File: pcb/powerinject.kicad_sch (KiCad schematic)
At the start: 3 parts, among them J1 PC_Usb, J2 Charger_USB, J3 Phone_USB

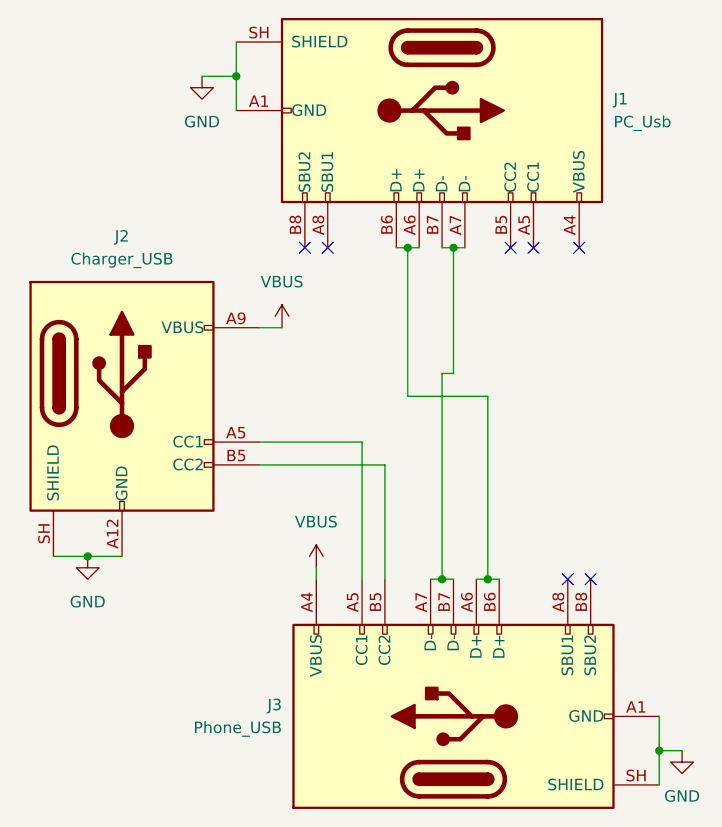
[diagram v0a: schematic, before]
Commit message: make pcb
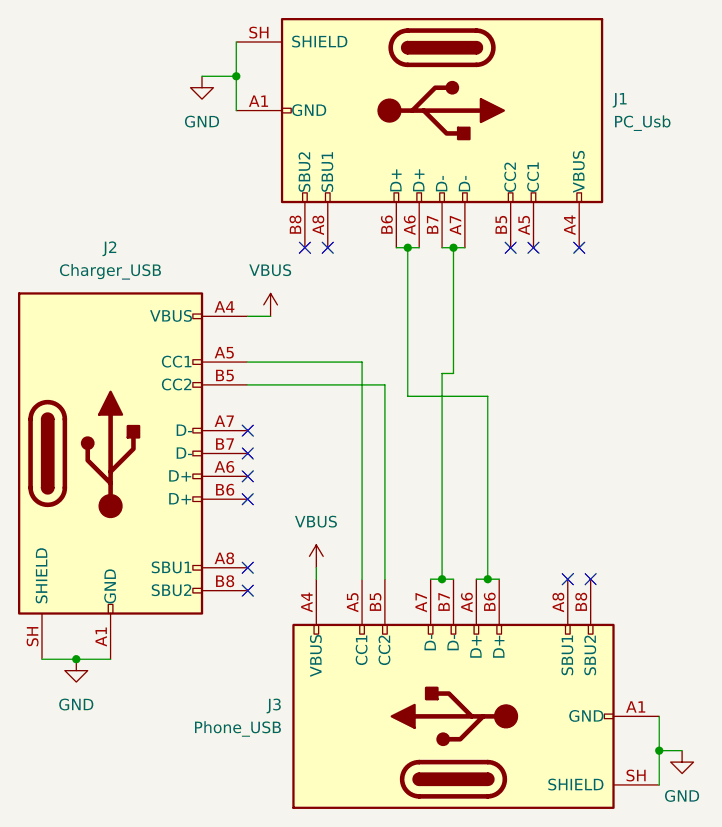
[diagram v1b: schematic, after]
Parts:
- J2: symbol Connector:USB_C_Receptacle_PowerOnly_6P -> Connector:USB_C_Receptacle_USB2.0_16P
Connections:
- net GND: now also J2.A1 (GND), J2.B1 (GND)
- net VBUS: now also J2.A4 (VBUS), J2.B4 (VBUS)
- no-connect marks 7 -> 13
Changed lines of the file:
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@@
+	)
+	(junction
+		(at 55.88 85.09)
+		(diameter 0)
+		(color 0 0 0 0)
 	)
 	(junction
@@
 		(color 0 0 0 0)
 	)
-	(junction
-		(at 57.15 73.66)
-		(diameter 0)
-		(color 0 0 0 0)
+	(no_connect
+		(at 74.93 62.23)
+	)
+	(no_connect
+		(at 74.93 64.77)
+	)
+	(no_connect
+		(at 74.93 77.47)
 	)
 	(no_connect
@@
 	)
 	(no_connect
+		(at 74.93 67.31)
+	)
+	(no_connect
 		(at 110.49 76.2)
 	)
@@
 	)
 	(no_connect
+		(at 74.93 59.69)
+	)
+	(no_connect
 		(at 104.14 39.37)
 	)
 	(no_connect
+		(at 74.93 74.93)
+	)
+	(no_connect
 		(at 106.68 39.37)
 	)
@@
 	(wire
 		(pts
-			(xy 53.34 73.66) (xy 57.15 73.66)
-		)
-		(stroke
-			(width 0)
-			(type default)
-		)
-	)
-	(wire
-		(pts
 			(xy 120.65 95.25) (xy 120.65 99.06)
 		)
@@
 	(wire
 		(pts
-			(xy 87.63 60.96) (xy 76.2 60.96)
-		)
-		(stroke
-			(width 0)
-			(type default)
-		)
-	)
-	(wire
-		(pts
-			(xy 90.17 63.5) (xy 76.2 63.5)
-		)
-		(stroke
-			(width 0)
-			(type default)
-		)
-	)
-	(wire
-		(pts
 			(xy 95.25 76.2) (xy 96.52 76.2)
 		)
@@
 	(wire
 		(pts
+			(xy 55.88 85.09) (xy 59.69 85.09)
+		)
+		(stroke
+			(width 0)
+			(type default)
+		)
+	)
+	(wire
+		(pts
 			(xy 101.6 55.88) (xy 101.6 76.2)
 		)
@@
 	(wire
 		(pts
+			(xy 74.93 46.99) (xy 77.47 46.99)
+		)
+		(stroke
+			(width 0)
+			(type default)
+		)
+	)
+	(wire
+		(pts
 			(xy 97.79 39.37) (xy 99.06 39.37)
 		)
@@
 	(wire
 		(pts
+			(xy 74.93 54.61) (xy 90.17 54.61)
+		)
+		(stroke
+			(width 0)
+			(type default)
+		)
+	)
+	(wire
+		(pts
 			(xy 73.66 16.51) (xy 73.66 20.32)
 		)
@@
 	(wire
 		(pts
-			(xy 76.2 48.26) (xy 78.74 48.26)
-		)
-		(stroke
-			(width 0)
-			(type default)
-		)
-	)
-	(wire
-		(pts
 			(xy 96.52 53.34) (xy 96.52 76.2)
 		)
@@
 	(wire
 		(pts
-			(xy 90.17 76.2) (xy 90.17 63.5)
+			(xy 90.17 54.61) (xy 90.17 76.2)
 		)
 		(stroke
@@
 	(wire
 		(pts
-			(xy 87.63 76.2) (xy 87.63 60.96)
-		)
-		(stroke
-			(width 0)
-			(type default)
-		)
-	)
-	(wire
-		(pts
-			(xy 57.15 73.66) (xy 60.96 73.66)
+			(xy 87.63 52.07) (xy 74.93 52.07)
+		)
+		(stroke
+			(width 0)
+			(type default)
+		)
+	)
+	(wire
+		(pts
+			(xy 87.63 52.07) (xy 87.63 76.2)
 		)
 		(stroke
@@
 		)
 	)
+	(wire
+		(pts
+			(xy 52.07 85.09) (xy 55.88 85.09)
+		)
+		(stroke
+			(width 0)
+			(type default)
+		)
+	)
 	(symbol
-		(lib_id "Connector:USB_C_Receptacle_PowerOnly_6P")
-		(at 60.96 55.88 0)
+		(lib_id "Connector:USB_C_Receptacle_USB2.0_16P")
+		(at 59.69 62.23 0)
 		(unit 1)
 		(body_style 1)
@@
 		(fields_autoplaced yes)
 		(property "Reference" "J2"
-			(at 60.96 38.1 0)
+			(at 59.69 39.37 0)
 			(show_name no)
 			(do_not_autoplace no)
@@
 		)
 		(property "Value" "Charger_USB"
-			(at 60.96 40.64 0)
+			(at 59.69 41.91 0)
 			(show_name no)
 			(do_not_autoplace no)
@@
 		)
 		(property "Footprint" "Connector_USB:USB_C_Receptacle_HRO_TYPE-C-31-M-12"
-			(at 64.77 53.34 0)
+			(at 63.5 62.23 0)
 			(hide yes)
 			(show_name no)
@@
 		)
 		(property "Datasheet" "https://www.usb.org/sites/default/files/documents/usb_type-c.zip"
-			(at 60.96 55.88 0)
-			(hide yes)
-			(show_name no)
-			(do_not_autoplace no)
-			(effects
-				(font
-					(size 1.27 1.27)
-				)
-			)
-		)
-		(property "Description" "USB Power-Only 6P Type-C Receptacle connector"
-			(at 60.96 55.88 0)
+			(at 63.5 62.23 0)
+			(hide yes)
+			(show_name no)
+			(do_not_autoplace no)
+			(effects
+				(font
+					(size 1.27 1.27)
+				)
+			)
+		)
+		(property "Description" "USB 2.0-only 16P Type-C Receptacle connector"
+			(at 59.69 62.23 0)
 			(hide yes)
 			(show_name no)
@@
 		)
 		(property "AliExpress Link" "https://pt.aliexpress.com/item/1005007419369264.html"
-			(at 60.96 55.88 0)
+			(at 59.69 62.23 0)
 			(hide yes)
 			(show_name no)
@@
 		)
 		(property "Price" "US $1.24"
-			(at 60.96 55.88 0)
+			(at 59.69 62.23 0)
 			(hide yes)
 			(show_name no)
@@
 		)
 		(pin "B12"
+		)
+		(pin "B6"
+		)
+		(pin "B8"
+		)
+		(pin "A6"
+		)
+		(pin "B1"
+		)
+		(pin "A1"
+		)
+		(pin "A4"
+		)
+		(pin "A7"
+		)
+		(pin "B7"
+		)
+		(pin "A8"
+		)
+		(pin "B4"
 		)
 		(instances
@@
 	(symbol
 		(lib_id "power:VBUS")
-		(at 78.74 48.26 0)
+		(at 77.47 46.99 0)
 		(unit 1)
 		(body_style 1)
@@
 		(fields_autoplaced yes)
 		(property "Reference" "#PWR02"
-			(at 78.74 52.07 0)
+			(at 77.47 50.8 0)
 			(hide yes)
 			(show_name no)
@@
 		)
 		(property "Value" "VBUS"
-			(at 78.74 43.18 0)
+			(at 77.47 41.91 0)
 			(show_name no)
 			(do_not_autoplace no)
@@
 		)
 		(property "Footprint" ""
-			(at 78.74 48.26 0)
+			(at 77.47 46.99 0)
 			(hide yes)
 			(show_name no)
@@
 		)
 		(property "Datasheet" ""
-			(at 78.74 48.26 0)
+			(at 77.47 46.99 0)
 			(hide yes)
 			(show_name no)
@@
 		)
 		(property "Description" "Power symbol creates a global label with name \"VBUS\""
-			(at 78.74 48.26 0)
+			(at 77.47 46.99 0)
 			(hide yes)
 			(show_name no)
@@
 	(symbol
 		(lib_id "power:GND")
-		(at 57.15 73.66 0)
+		(at 55.88 85.09 0)
 		(unit 1)
 		(body_style 1)
@@
 		(fields_autoplaced yes)
 		(property "Reference" "#PWR03"
-			(at 57.15 80.01 0)
+			(at 55.88 91.44 0)
 			(hide yes)
 			(show_name no)
@@
 		)
 		(property "Value" "GND"
-			(at 57.15 78.74 0)
+			(at 55.88 90.17 0)
 			(show_name no)
 			(do_not_autoplace no)
@@
 		)
 		(property "Footprint" ""
-			(at 57.15 73.66 0)
+			(at 55.88 85.09 0)
 			(hide yes)
 			(show_name no)
@@
 		)
 		(property "Datasheet" ""
-			(at 57.15 73.66 0)
+			(at 55.88 85.09 0)
 			(hide yes)
 			(show_name no)
@@
 		)
 		(property "Description" "Power symbol creates a global label with name \"GND\" , ground"
-			(at 57.15 73.66 0)
-			(hide yes)
-			(show_name no)
+			(at 55.88 85.09 0)
+			(hide yes)
+			(show_name no)
